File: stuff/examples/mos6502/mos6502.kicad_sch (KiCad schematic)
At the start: 15 parts, among them U1 Mos6532

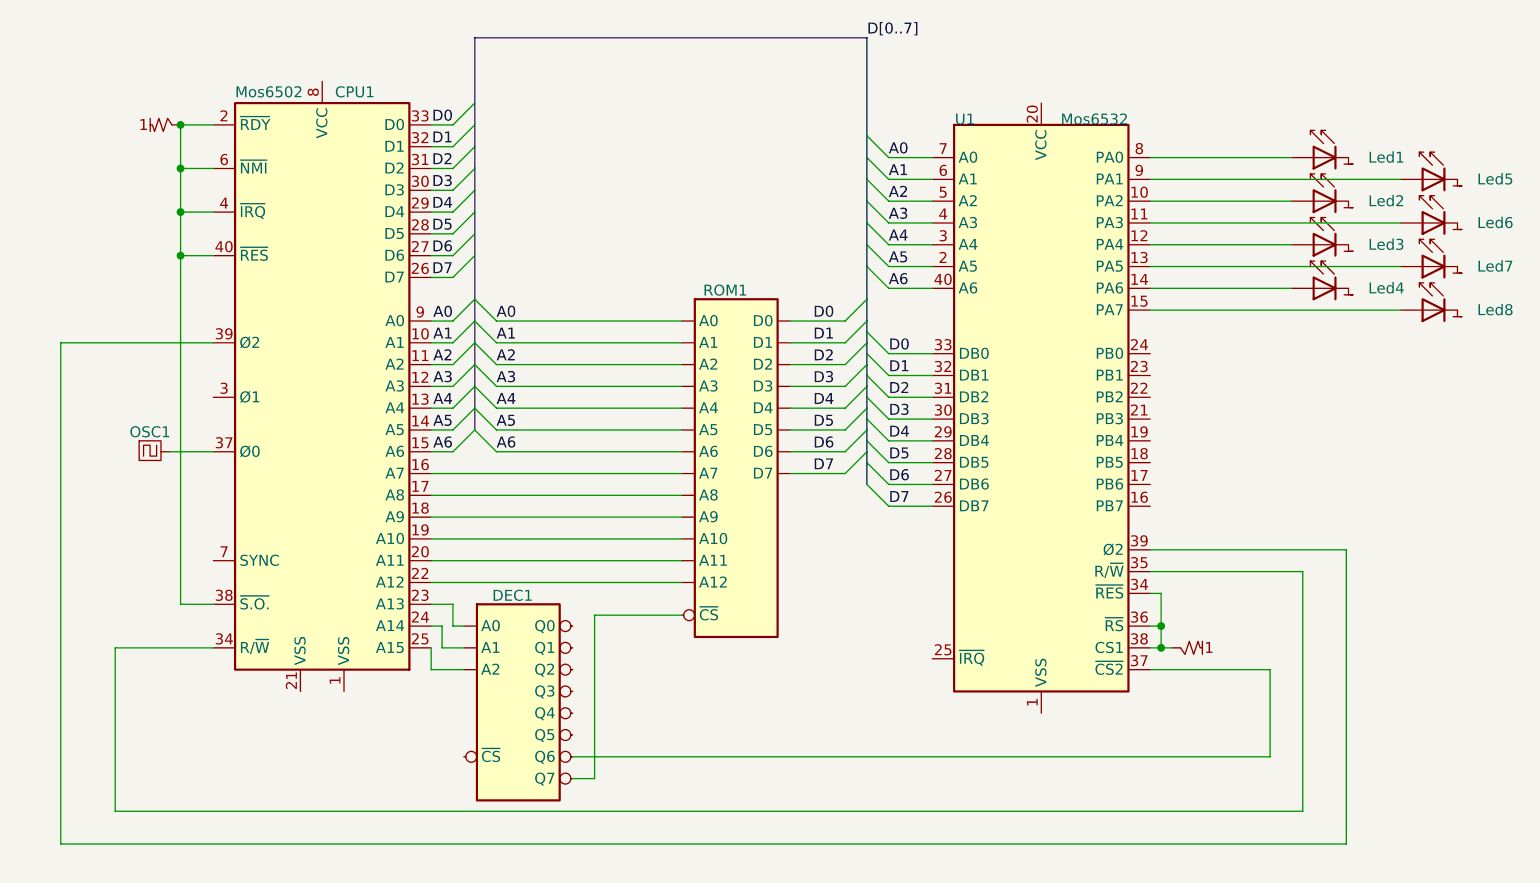
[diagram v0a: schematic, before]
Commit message: Mos6502/6532 - example
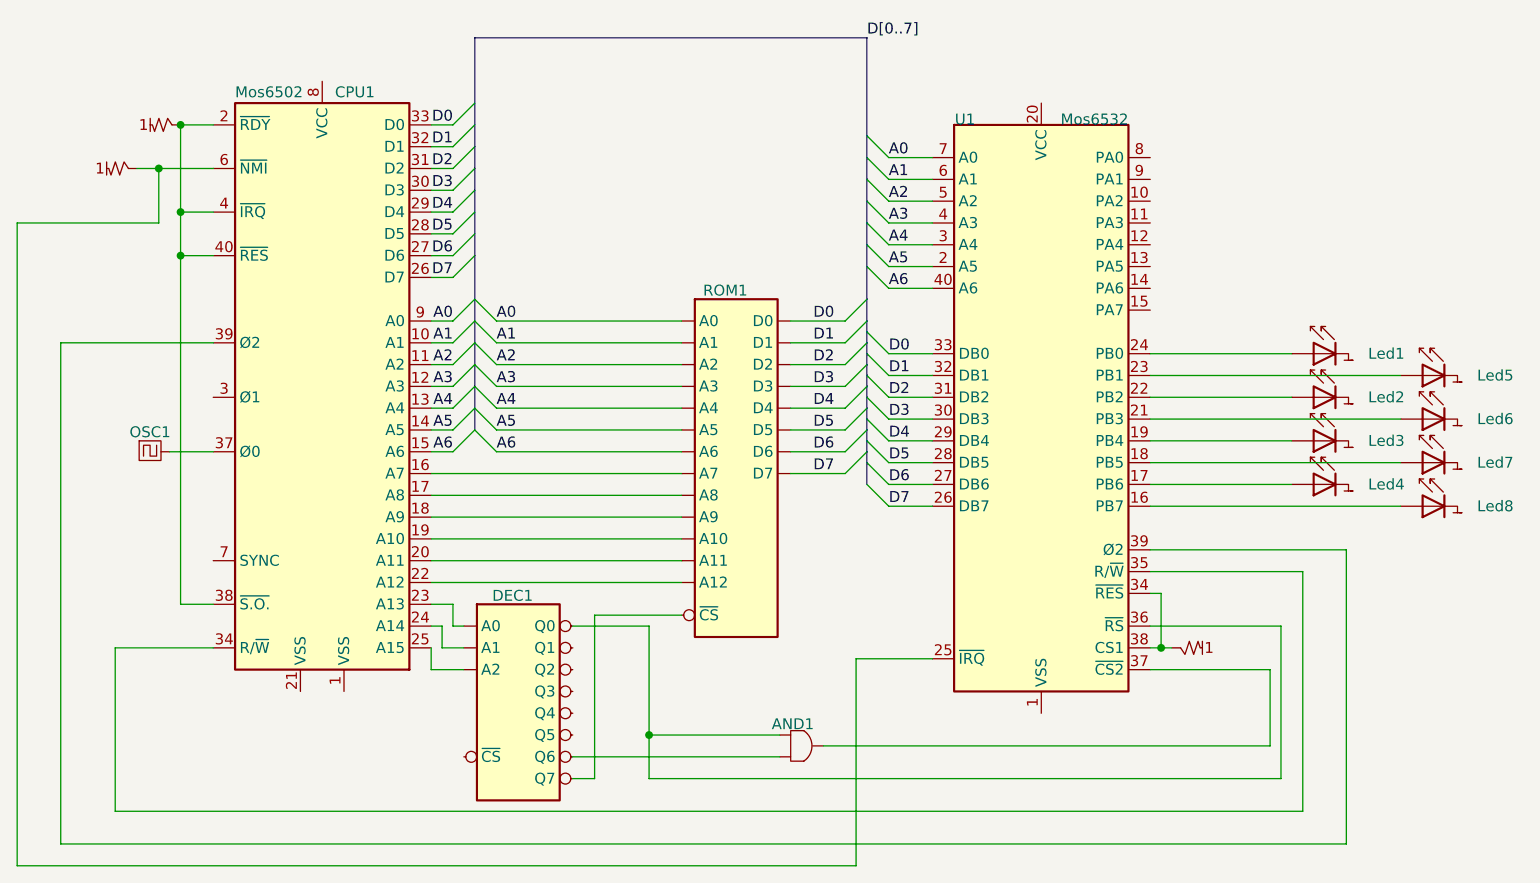
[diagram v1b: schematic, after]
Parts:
- added AND1: AND, symbol chip:AND
- added pullup3: pull_up, symbol chip:PULLUP
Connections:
- net at Led2.1 (IN): now also U1.22 (PB2); no longer U1.10 (PA2)
- net at Led8.1 (IN): now also U1.16 (PB7); no longer U1.15 (PA7)
- net at U1.34 (~{RES}), U1.38 (CS1), pullup2.1 (OUT): no longer U1.36 (~{RS})
- net at CPU1.2 (~{RDY}), CPU1.38 (~{S.O.}), CPU1.4 (~{IRQ})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: no longer CPU1.6 (~{NMI})
- net at Led4.1 (IN): now also U1.17 (PB6); no longer U1.14 (PA6)
- net at Led5.1 (IN): now also U1.23 (PB1); no longer U1.9 (PA1)
- net at Led6.1 (IN): now also U1.21 (PB3); no longer U1.11 (PA3)
- net at DEC1.10 (Q6): now also AND1.2 (IN1); no longer U1.37 (~{CS2})
- net at DEC1.4 (Q0): now also U1.36 (~{RS}), AND1.1 (IN0)
- net at Led3.1 (IN): now also U1.19 (PB4); no longer U1.12 (PA4)
- net at Led7.1 (IN): now also U1.18 (PB5); no longer U1.13 (PA5)
- net at U1.24 (PB0): now also Led1.1 (IN)
- net at U1.25 (~{IRQ}): now also CPU1.6 (~{NMI}), pullup3.1 (OUT)
- net at U1.8 (PA0): no longer Led1.1 (IN)
- new net: AND1.3 (OUT), U1.37 (~{CS2})
